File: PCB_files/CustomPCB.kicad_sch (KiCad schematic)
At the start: 7 parts, among them J1 Conn_01x04_Socket, J2 Conn_01x01_Socket, J3 Conn_01x01_Socket, J4 Barrel_Jack_MountingPin

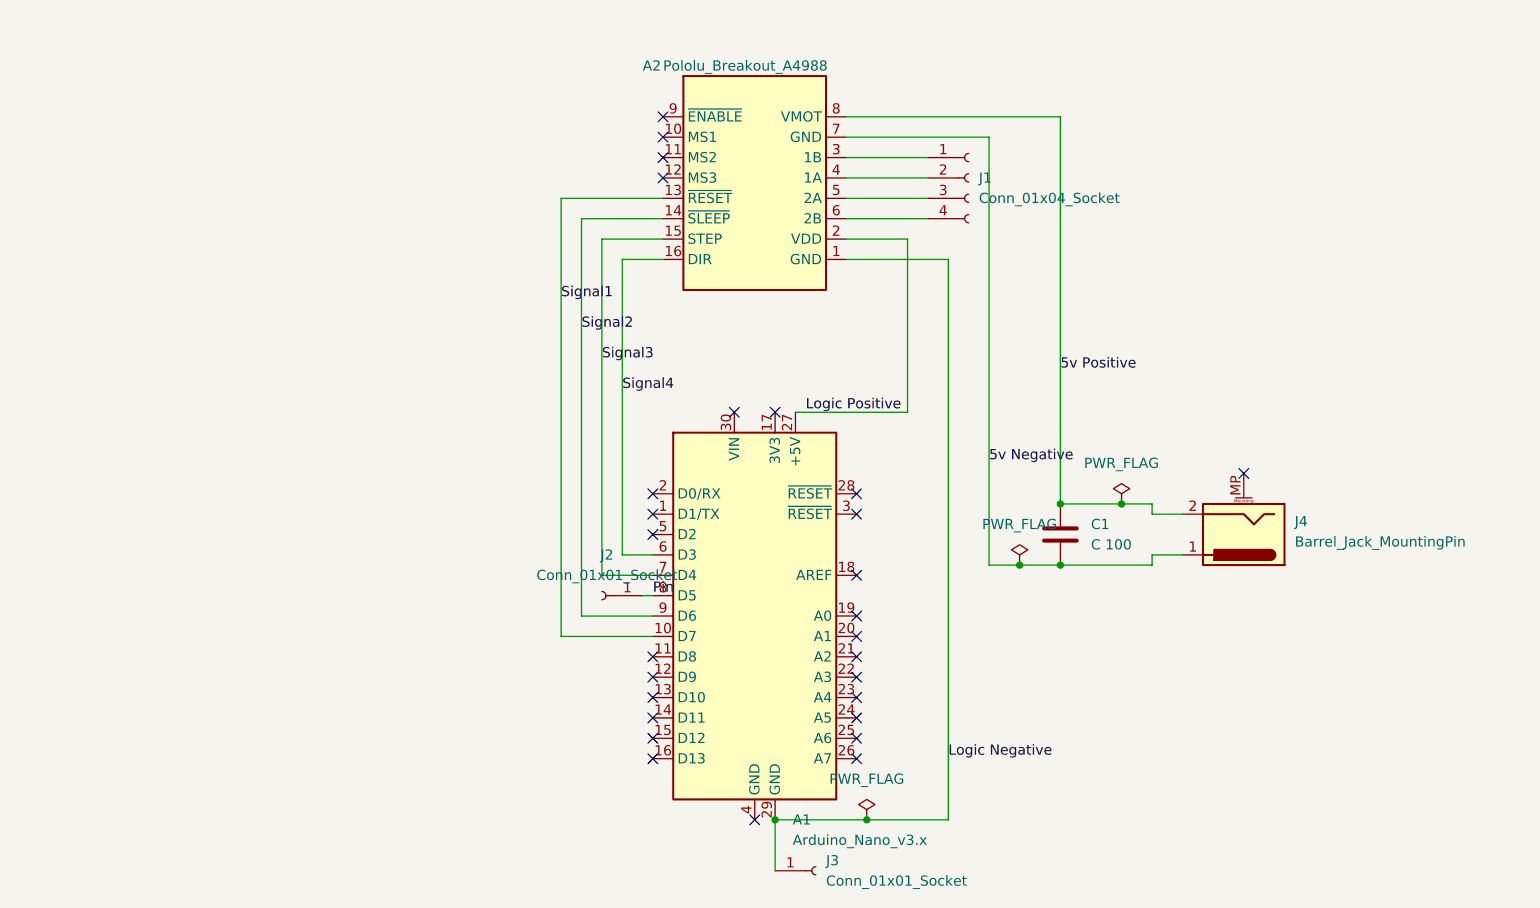
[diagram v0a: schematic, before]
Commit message: PCB V2
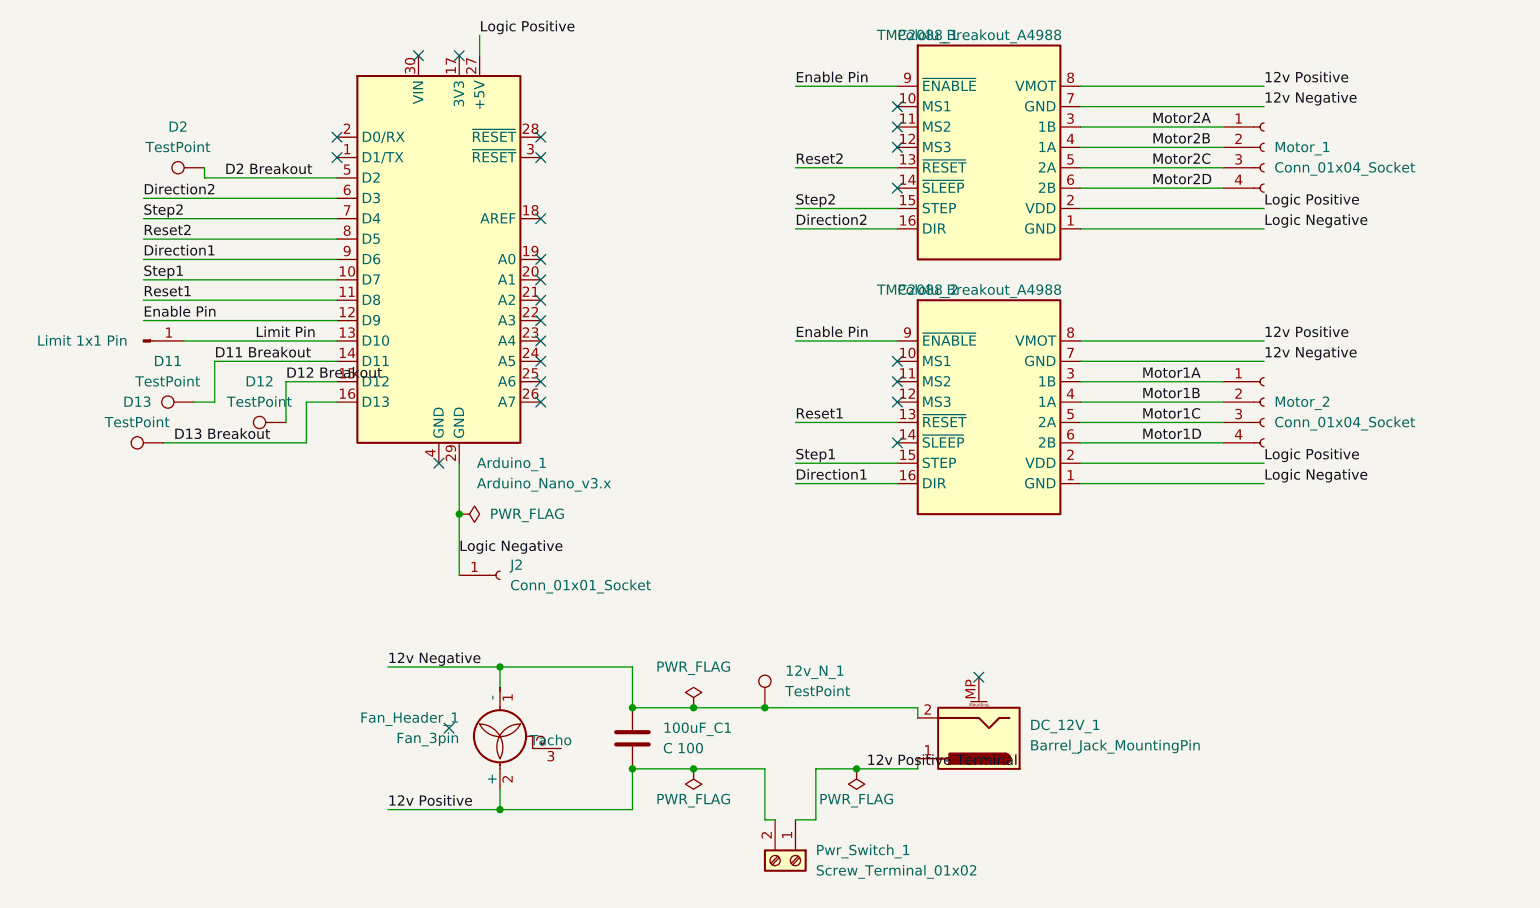
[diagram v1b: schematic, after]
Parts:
- added 12v_N_1, D11, D12, D13, D2: TestPoint, TestPoint:TestPoint_Pad_1.5x1.5mm, symbol Connector:TestPoint
- added Fan_Header_1: Fan_3pin, Connector:FanPinHeader_1x03_P2.54mm_Vertical, symbol Motor:Fan_3pin
- added Motor_1: Conn_01x04_Socket, Connector_PinSocket_2.54mm:PinSocket_1x04_P2.54mm_Vertical, symbol Connector:Conn_01x04_Socket
- added Pwr_Switch_1: Screw_Terminal_01x02, TerminalBlock:TerminalBlock_bornier-2_P5.08mm, symbol Connector:Screw_Terminal_01x02
- added TMC2088_1: Pololu_Breakout_A4988, Module:Pololu_Breakout-16_15.2x20.3mm, symbol Driver_Motor:Pololu_Breakout_A4988
- J1: renamed from J2; value Conn_01x01_Socket -> Limit 1x1 Pin; footprint Connector_PinSocket_2.54mm:PinSocket_1x01_P2.54mm_Vertical -> Connector_PinHeader_2.54mm:PinHeader_1x01_P2.54mm_Vertical; symbol Connector:Conn_01x01_Socket -> Connector:Conn_01x01_Pin
- J2: renamed from J3; footprint Connector_PinSocket_2.54mm:PinSocket_1x01_P2.54mm_Vertical -> Connector_PinHeader_2.54mm:PinHeader_1x01_P2.54mm_Vertical
- renumbered C1 to 100uF_C1, A1 to Arduino_1, J4 to DC_12V_1, J1 to Motor_2, A2 to TMC2088_2
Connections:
- net Logic Negative: now also TMC2088_1.1 (GND)
- net Logic Positive: now also TMC2088_1.2 (VDD)
- net Motor1A: now reaches Motor_2.1 (Pin_1), TMC2088_2.3 (1B)
- net Motor1B: now reaches Motor_2.2 (Pin_2), TMC2088_2.4 (1A)
- net Motor1C: now reaches Motor_2.3 (Pin_3), TMC2088_2.5 (2A)
- net Motor1D: now reaches Motor_2.4 (Pin_4), TMC2088_2.6 (2B)
- net Reset1: now reaches Arduino_1.11 (D8)
- net Reset1: now also TMC2088_2.13 (~{RESET})
- net Enable Pin: now reaches Arduino_1.12 (D9)
- net Enable Pin: now also TMC2088_2.9 (~{ENABLE}), TMC2088_1.9 (~{ENABLE})
- net Limit Pin: now reaches Arduino_1.13 (D10)
- net Limit Pin: now also J1.1 (Pin_1)
- net D11 Breakout: now reaches Arduino_1.14 (D11)
- net D11 Breakout: now also D11.1
- net D12 Breakout: now reaches Arduino_1.15 (D12)
- net D12 Breakout: now also D12.1
- net D13 Breakout: now reaches Arduino_1.16 (D13)
- net D13 Breakout: now also D13.1
- net D2 Breakout: now reaches Arduino_1.5 (D2)
- net D2 Breakout: now also D2.1
- removed net 5v Negative: 100uF_C1.1, DC_12V_1.1, TMC2088_2.7 (GND)
- net 5v Positive renamed 12v Negative
- net 12v Negative: now also TMC2088_2.7 (GND), 12v_N_1.1, Fan_Header_1.1 (-), TMC2088_1.7 (GND); no longer TMC2088_2.8 (VMOT)
- net Pin renamed Reset2
- net Reset2: now also TMC2088_1.13 (~{RESET}); no longer J1.1 (Pin_1)
- net Signal1 renamed Step1
- net Step1: now also TMC2088_2.15 (STEP); no longer TMC2088_2.13 (~{RESET})
- net Signal2: no longer names the net of TMC2088_2.14 (~{SLEEP})
- net Signal2: no longer Arduino_1.9 (D6)
- net Signal3 renamed Step2
- net Step2: now also TMC2088_1.15 (STEP); no longer TMC2088_2.15 (STEP)
- net Signal4 renamed Direction1
- net Direction1: now also Arduino_1.9 (D6); no longer Arduino_1.6 (D3)
- new net 12v Positive: 100uF_C1.1, Fan_Header_1.2 (+), Pwr_Switch_1.2 (Pin_2), TMC2088_1.8 (VMOT), TMC2088_2.8 (VMOT)
- new net 12v Positive Terminal: DC_12V_1.1, Pwr_Switch_1.1 (Pin_1)
- new net Direction2: Arduino_1.6 (D3), TMC2088_1.16 (DIR)
- new net Motor2A: Motor_1.1 (Pin_1), TMC2088_1.3 (1B)
- new net Motor2B: Motor_1.2 (Pin_2), TMC2088_1.4 (1A)
- new net Motor2C: Motor_1.3 (Pin_3), TMC2088_1.5 (2A)
- new net Motor2D: Motor_1.4 (Pin_4), TMC2088_1.6 (2B)
- no-connect marks 28 -> 26
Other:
- moved on the sheet: 100uF_C1, Arduino_1, DC_12V_1, J2, Motor_2, TMC2088_2
